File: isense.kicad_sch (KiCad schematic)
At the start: 29 parts, among them U1 MAX4073T, U2 OPA551U, U3 TLV9301xDBV, U4 OPA551U, U5 TLV9301xDBV

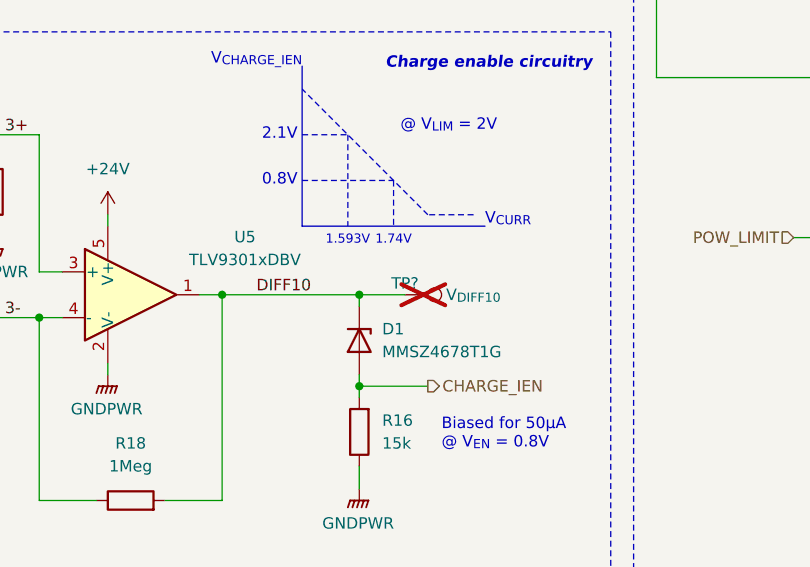
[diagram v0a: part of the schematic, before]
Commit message: Completed preliminary layout
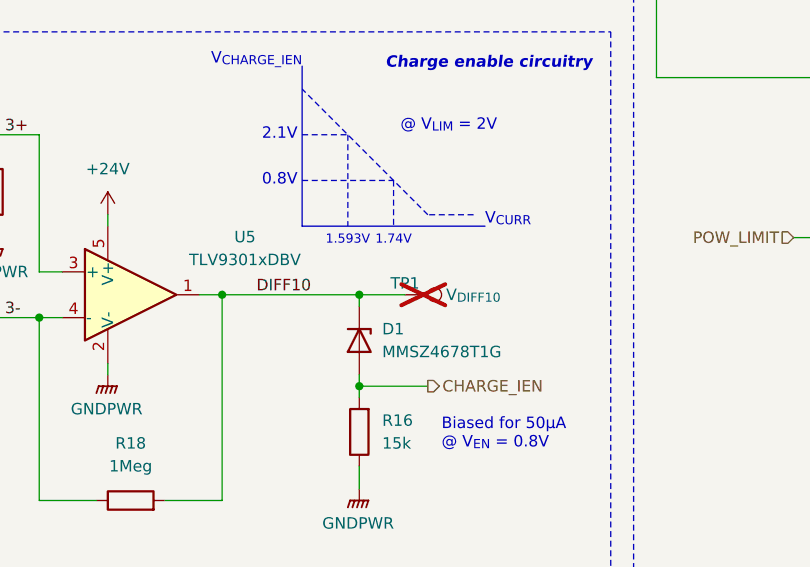
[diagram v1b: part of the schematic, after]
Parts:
- gave numbers to parts that had none: 1
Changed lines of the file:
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@@
 		(dnp no)
 		(fields_autoplaced yes)
-		(property "Reference" "#PWR019"
+		(property "Reference" "#PWR040"
 			(at 96.52 52.07 0)
 			(effects
@@
 		(dnp no)
 		(fields_autoplaced yes)
-		(property "Reference" "#PWR033"
+		(property "Reference" "#PWR054"
 			(at 158.75 140.97 0)
 			(effects
@@
 		(on_board yes)
 		(dnp yes)
-		(property "Reference" "TP?"
+		(property "Reference" "TP1"
 			(at 163.83 113.03 90)
 			(effects
@@
 		(dnp no)
 		(fields_autoplaced yes)
-		(property "Reference" "#PWR022"
+		(property "Reference" "#PWR043"
 			(at 132.08 69.85 0)
 			(effects
@@
 		(dnp no)
 		(fields_autoplaced yes)
-		(property "Reference" "#PWR029"
+		(property "Reference" "#PWR050"
 			(at 118.11 113.03 0)
 			(effects
@@
 		(dnp no)
 		(fields_autoplaced yes)
-		(property "Reference" "#PWR027"
+		(property "Reference" "#PWR048"
 			(at 223.52 106.68 0)
 			(effects
@@
 		(dnp no)
 		(fields_autoplaced yes)
-		(property "Reference" "#PWR018"
+		(property "Reference" "#PWR039"
 			(at 54.61 52.07 0)
 			(effects
@@
 		(dnp no)
 		(fields_autoplaced yes)
-		(property "Reference" "#PWR023"
+		(property "Reference" "#PWR044"
 			(at 181.61 71.12 0)
 			(effects
@@
 		(dnp no)
 		(fields_autoplaced yes)
-		(property "Reference" "#PWR017"
+		(property "Reference" "#PWR038"
 			(at 223.52 50.8 0)
 			(effects
@@
 		(dnp no)
 		(fields_autoplaced yes)
-		(property "Reference" "#PWR021"
+		(property "Reference" "#PWR042"
 			(at 181.61 53.34 0)
 			(effects
@@
 		(dnp no)
 		(fields_autoplaced yes)
-		(property "Reference" "#PWR020"
+		(property "Reference" "#PWR041"
 			(at 132.08 53.34 0)
 			(effects
@@
 		(dnp no)
 		(fields_autoplaced yes)
-		(property "Reference" "#PWR028"
+		(property "Reference" "#PWR049"
 			(at 130.81 109.22 0)
 			(effects
@@
 		(dnp no)
 		(fields_autoplaced yes)
-		(property "Reference" "#PWR034"
+		(property "Reference" "#PWR055"
 			(at 243.84 143.51 0)
 			(effects
@@
 		(dnp no)
 		(fields_autoplaced yes)
-		(property "Reference" "#PWR025"
+		(property "Reference" "#PWR046"
 			(at 243.84 87.63 0)
 			(effects
@@
 		(dnp no)
 		(fields_autoplaced yes)
-		(property "Reference" "#PWR016"
+		(property "Reference" "#PWR037"
 			(at 243.84 44.45 0)
 			(effects
@@
 		(dnp no)
 		(fields_autoplaced yes)
-		(property "Reference" "#PWR030"
+		(property "Reference" "#PWR051"
 			(at 130.81 128.27 0)
 			(effects
@@
 		(dnp no)
 		(fields_autoplaced yes)
-		(property "Reference" "#PWR026"
+		(property "Reference" "#PWR047"
 			(at 243.84 100.33 0)
 			(effects
@@
 		(dnp no)
 		(fields_autoplaced yes)
-		(property "Reference" "#PWR032"
+		(property "Reference" "#PWR053"
 			(at 93.98 140.97 0)
 			(effects
@@
 		(dnp no)
 		(fields_autoplaced yes)
-		(property "Reference" "#PWR024"
+		(property "Reference" "#PWR045"
 			(at 96.52 71.12 0)
 			(effects
@@
 		(dnp no)
 		(fields_autoplaced yes)
-		(property "Reference" "#PWR031"
+		(property "Reference" "#PWR052"
 			(at 93.98 129.54 0)
 			(effects
